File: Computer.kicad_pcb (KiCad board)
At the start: 2 copper layers, 35 parts, among them J1 DB9, J2 Screw_Terminal_1x04, U1 8284, U10 74LS04, U11 7400, U12 8259, U2 LM2931AZ-5.0, U3 8088, U4 74LS04, U5 28C256, U6 RAM_32KO, U7 16450, U8 7400, U9 NCP1117DT12G, Y1 8 MHz, Y2 3.072 MHz

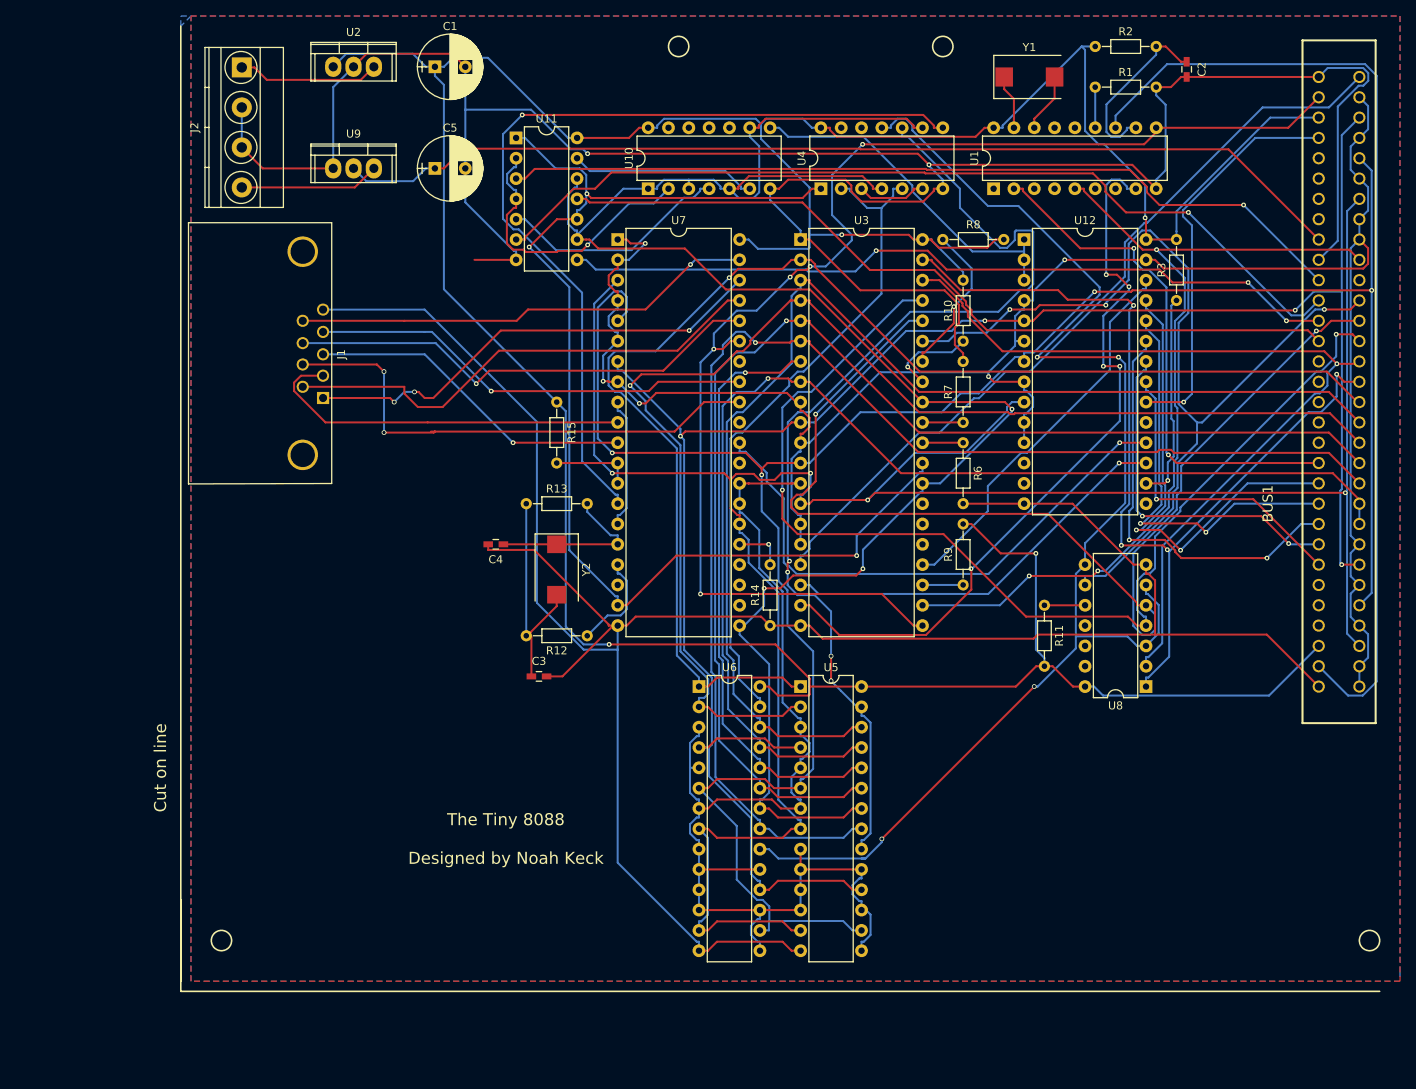
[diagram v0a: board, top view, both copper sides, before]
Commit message: Update to revision A
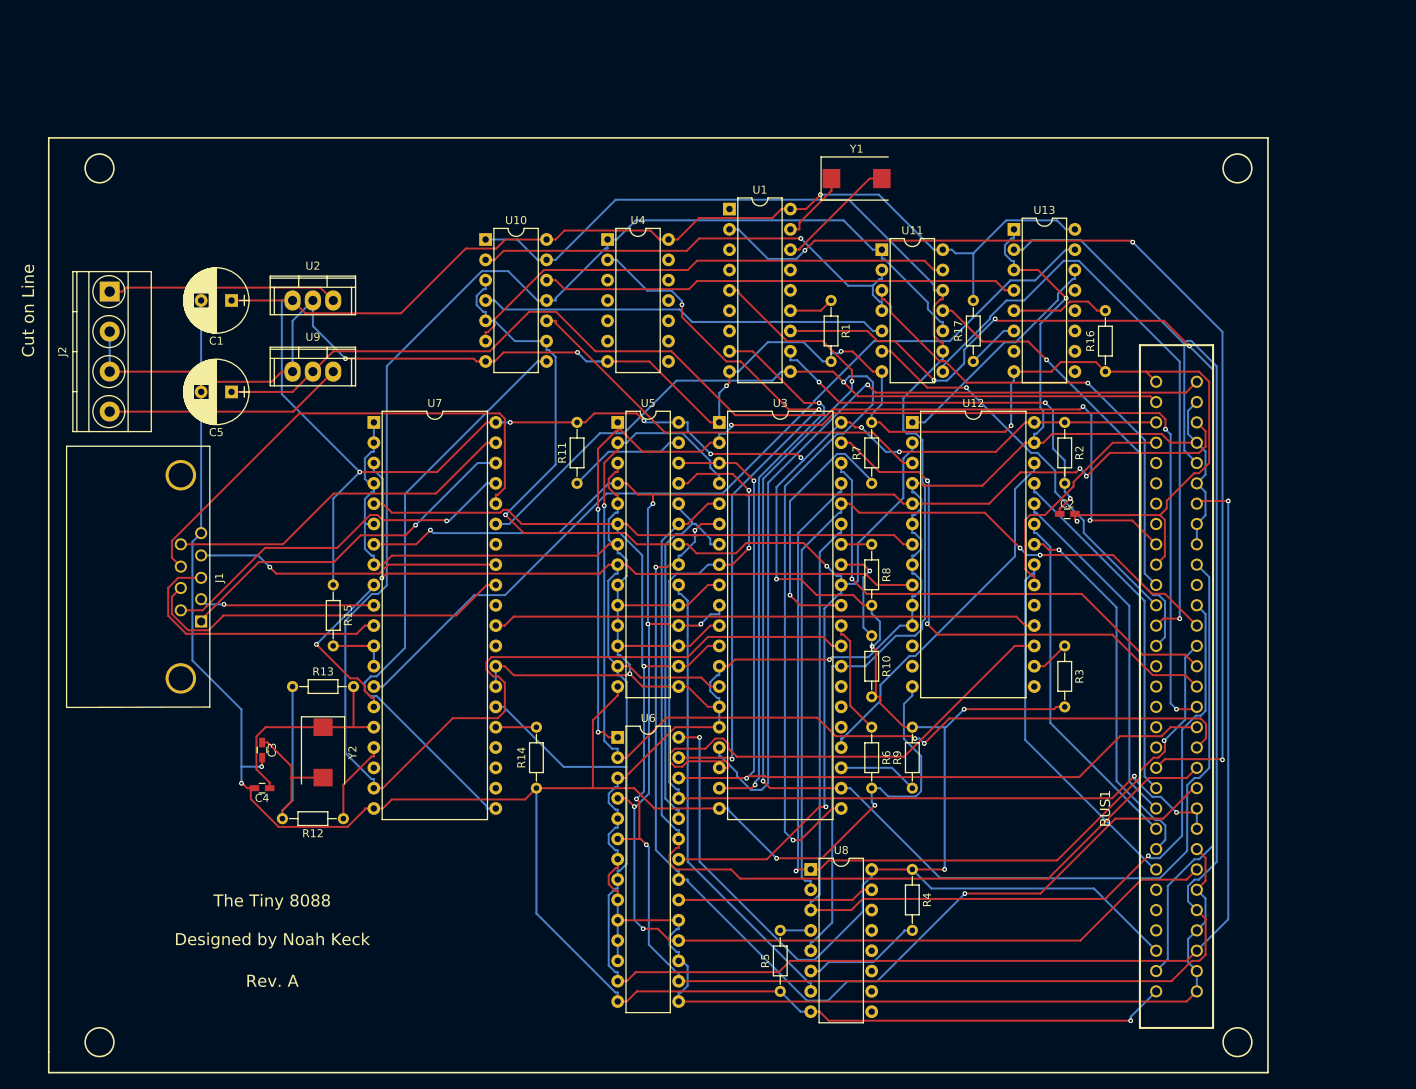
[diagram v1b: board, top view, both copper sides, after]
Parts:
- added R16: 10k, Resistors_THT:R_Axial_DIN0204_L3.6mm_D1.6mm_P7.62mm_Horizontal, F.Cu at (163.8, 57.1)
- added R17: 10k, Resistors_THT:R_Axial_DIN0204_L3.6mm_D1.6mm_P7.62mm_Horizontal, F.Cu at (147.3, 55.9)
- added R4: 10k, Resistors_THT:R_Axial_DIN0204_L3.6mm_D1.6mm_P7.62mm_Horizontal, F.Cu at (139.7, 119.4)
- added R5: 10k, Resistors_THT:R_Axial_DIN0204_L3.6mm_D1.6mm_P7.62mm_Horizontal, F.Cu at (123.2, 134.6)
- added U13: 74LS138, Housings_DIP:DIP-16_W7.62mm, F.Cu at (152.4, 39.4)
- U8: value 7400 -> 74LS138; footprint Housings_DIP:DIP-14_W7.62mm -> Housings_DIP:DIP-16_W7.62mm
- moved R11 60.4 mm to (97.8, 71.1), turned to 90 degrees
- moved C2 57.5 mm to (159.1, 74.9), turned to 0 degrees
- moved U11 47.8 mm to (135.9, 41.9)
- moved U8 47.7 mm to (127.0, 119.4), turned to 0 degrees
- moved R2 47.1 mm to (158.8, 63.5), turned to 270 degrees
- moved R3 45.4 mm to (158.8, 91.4), turned to 270 degrees
- moved BUS1 43.2 mm to (172.7, 123.2)
- moved R1 42.4 mm to (129.5, 48.3), turned to 270 degrees
- moved C4 42.2 mm to (58.4, 109.2)
- moved U5 40.2 mm to (102.9, 63.5)
- moved R8 39.1 mm to (134.6, 78.7), turned to 270 degrees
- moved C1 38.7 mm to (54.6, 48.3), turned to 180 degrees
- moved R10 38.6 mm to (134.6, 90.2), turned to 270 degrees
- moved R12 38.1 mm to (68.6, 113.0)
- moved U7 38.1 mm to (72.4, 63.5)
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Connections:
- U10 pad 10: (no net) -> Net-(U10-Pad10)
- U10 pad 11: (no net) -> WR
- U10 pad 12: (no net) -> Net-(U10-Pad12)
- U10 pad 13: (no net) -> IO/M
- U10 pad 3: IO/M -> RD
- U10 pad 5: IO/M -> RD
- U10 pad 9: IO/M -> RD
- U12 pad 1: Net-(U10-Pad8) -> Net-(U12-Pad1)
- U12 pad 2: Net-(U10-Pad8) -> RD
- U12 pad 3: Net-(U10-Pad8) -> Net-(U10-Pad10)
- U3 pad 32: IO/M -> RD
- U4 pad 10: Net-(U4-Pad10) -> (no net)
- U4 pad 11: Net-(U4-Pad11) -> (no net)
- U4 pad 3: Net-(U4-Pad3) -> (no net)
- U4 pad 4: IO/M -> (no net)
- U4 pad 5: Net-(U4-Pad2) -> (no net)
- U4 pad 6: Net-(U4-Pad3) -> (no net)
- U4 pad 8: Net-(U4-Pad8) -> (no net)
- U4 pad 9: IO/M -> (no net)
- U5 pad 20: Net-(U4-Pad10) -> Net-(U5-Pad20)
- U5 pad 22: IO/M -> RD
- U5 pad 27: Net-(U4-Pad10) -> Net-(R11-Pad1)
- U6 pad 20: Net-(U4-Pad11) -> Net-(U6-Pad20)
- U6 pad 22: IO/M -> RD
- U7 pad 14: Net-(U4-Pad8) -> Net-(U13-Pad15)
- U7 pad 21: IO/M -> Net-(U10-Pad8)
- U8 pad 1: A15 -> A17
- U8 pad 10: Net-(R11-Pad1) -> Net-(U8-Pad10)
- U8 pad 11: (no net) -> Net-(U8-Pad11)
- U8 pad 12: (no net) -> Net-(U8-Pad12)
- U8 pad 13: (no net) -> Net-(U8-Pad13)
- U8 pad 14: Vcc -> Net-(U8-Pad14)
- U8 pad 2: A16 -> A18
- U8 pad 3: Net-(U4-Pad11) -> A19
- U8 pad 4: A17 -> Net-(R5-Pad2)
- U8 pad 5: A18 -> IO/M
- U8 pad 6: Net-(U4-Pad11) -> Net-(R4-Pad2)
- U8 pad 7: GND -> Net-(U5-Pad20)
- U8 pad 8: Net-(U4-Pad11) -> GND
- U8 pad 9: A19 -> Net-(U8-Pad9)
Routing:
- net Net-(U4-Pad11): track 168.3 -> 0.00 mm, vias 4 -> 0
- net RD: track 0.00 -> 159.7 mm, vias 0 -> 3
- net Net-(U4-Pad10): track 131.0 -> 0.00 mm, vias 4 -> 0
- net Net-(U13-Pad15): track 0.00 -> 110.3 mm
- net Net-(U4-Pad8): track 109.5 -> 0.00 mm, vias 1 -> 0
- net IO/M: track 240.1 -> 164.1 mm, vias 3 -> 0
- net WR: track 151.4 -> 219.4 mm, vias 3 -> 0
- net Net-(BUS1-Pad20): track 65.5 -> 131.1 mm, vias 2 -> 3
- net GND: track 589.6 -> 526.7 mm, vias 2 -> 11
- net Net-(BUS1-Pad41): track 110.0 -> 172.9 mm, vias 3 -> 2
- net Net-(BUS1-Pad12): track 112.6 -> 49.9 mm
- net Net-(U10-Pad12): track 0.00 -> 59.8 mm
- net Net-(U5-Pad20): track 0.00 -> 58.0 mm
- net A4: track 282.2 -> 336.1 mm, vias 4 -> 3
- net Net-(U10-Pad10): track 0.00 -> 53.2 mm
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- removed copper zone on B.Cu, net GND
- removed copper zone on F.Cu, net Vcc
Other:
- board text added: "Cut on Line"
- board text added: "Rev. A"
- board text removed: "Cut on line"
